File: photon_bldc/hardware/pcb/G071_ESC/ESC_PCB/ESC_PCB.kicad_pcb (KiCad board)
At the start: 4 copper layers, 36 x 16 mm, 69 parts, among them J2 Plus, J3 Minus, Q1 NMOS, Q2 NMOS, Q3 NMOS, Q4 NMOS, Q5 NMOS, Q6 NMOS, U1 STM32G071GBUx, U4 L78L06_SOT89

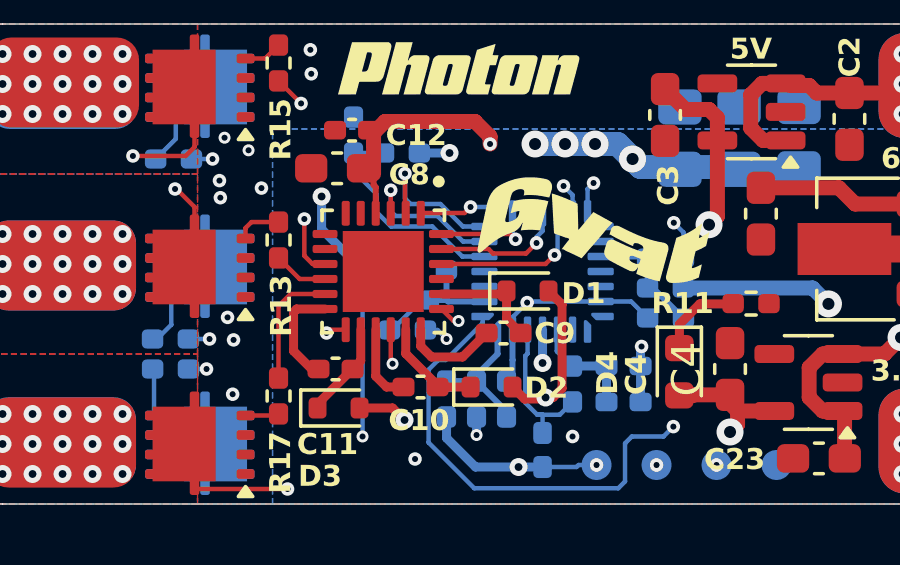
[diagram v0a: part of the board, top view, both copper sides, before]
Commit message: 11.05.2025r
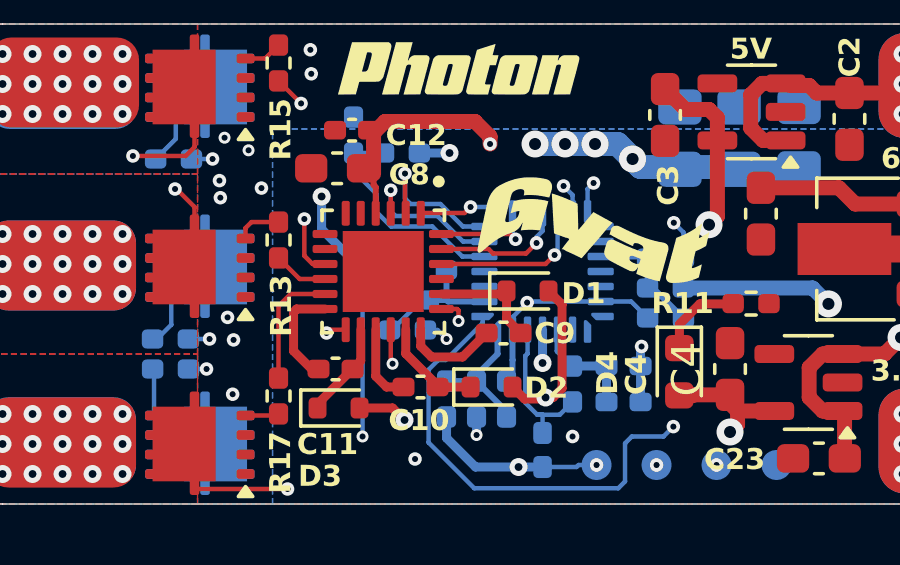
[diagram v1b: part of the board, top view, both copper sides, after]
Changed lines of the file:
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@@
 	)
 	(segment
-		(start 87.2 53.9)
-		(end 87.03 53.9)
+		(start 87.2 53.55)
+		(end 87.15 53.5)
 		(width 0.15)
 		(layer "F.Cu")
@@
 	)
 	(segment
-		(start 87.03 53.9)
+		(start 87.2 53.9)
+		(end 87.2 53.55)
+		(width 0.15)
+		(layer "F.Cu")
+		(net 14)
+	)
+	(segment
+		(start 87.15 53.5)
 		(end 86.63 53.5)
 		(width 0.15)

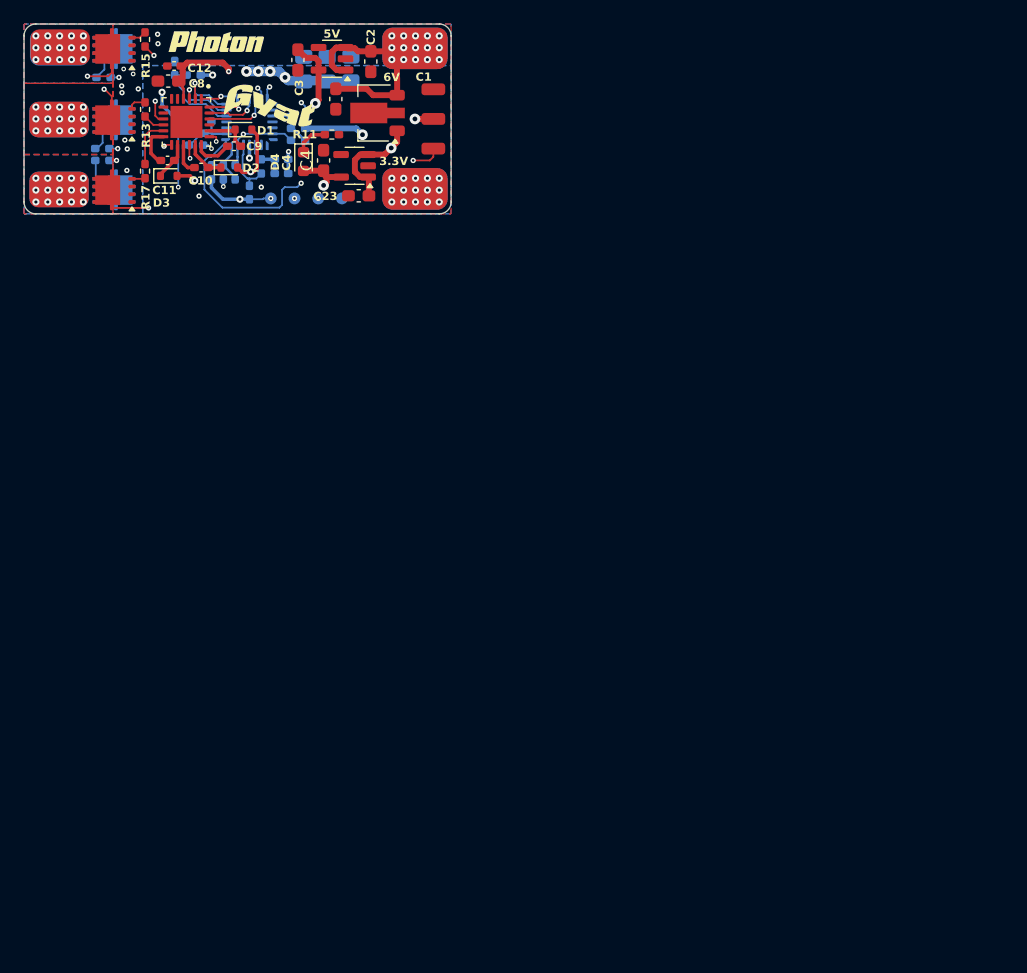
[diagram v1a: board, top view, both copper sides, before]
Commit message: esc
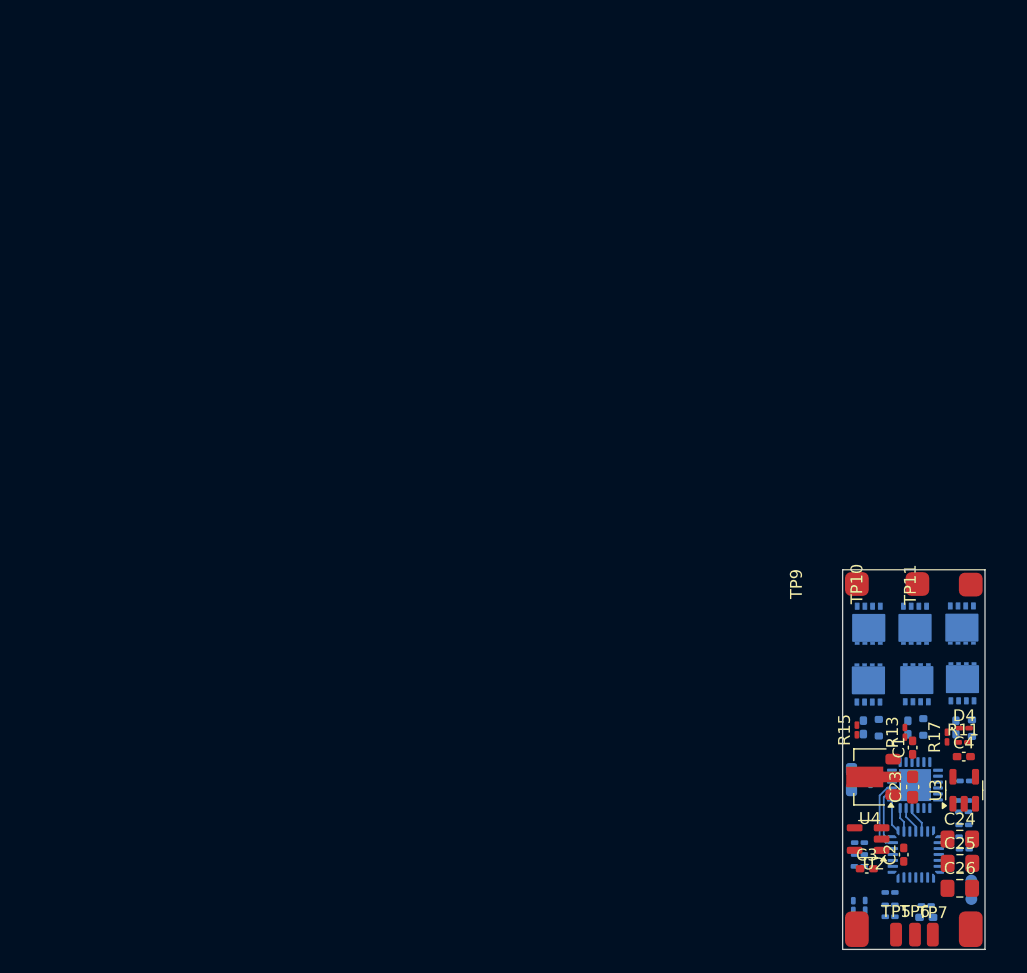
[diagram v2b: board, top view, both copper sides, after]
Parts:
- removed ? (x5): , 
- removed C5: 100nF, Capacitor_SMD:C_0402_1005Metric_Pad0.74x0.62mm_HandSolder
- removed G*** (x2): LOGO, LOGO
- removed R2: 10k, Resistor_SMD:R_0402_1005Metric_Pad0.72x0.64mm_HandSolder
- C1, C2, C3, C4: footprint Capacitor_SMD:C_0603_1608Metric_Pad1.08x0.95mm_HandSolder -> Capacitor_SMD:C_0402_1005Metric_Pad0.74x0.62mm_HandSolder
- C10, C11, C8, C9, D1, D2, D3, U6: moved to B.Cu
- C12: footprint Capacitor_SMD:C_0402_1005Metric_Pad0.74x0.62mm_HandSolder -> Capacitor_SMD:C_0201_0603Metric_Pad0.64x0.40mm_HandSolder; moved to B.Cu
- C24, C25, C26: moved to F.Cu
- C6: footprint Capacitor_SMD:C_0402_1005Metric_Pad0.74x0.62mm_HandSolder -> Capacitor_SMD:C_0201_0603Metric_Pad0.64x0.40mm_HandSolder
- D4: footprint LED_SMD:LED_0603_1608Metric -> LED_SMD:LED_0201_0603Metric_Pad0.64x0.40mm_HandSolder
- Q1, Q2, Q3: footprint Fortior Tech FD6288Q driver library:TSON-8(3.1x3.1) -> MOSFET_lib:NCEP3065
- Q4, Q5, Q6: footprint Fortior Tech FD6288Q driver library:TSON-8(3.1x3.1) -> MOSFET_lib:NCEP3065; moved to B.Cu
- R1, R10, R11, R12, R13, R14, R15, R16, R17, R18, R19, R3, R4, R5, R6, R7, R8, R9: footprint Resistor_SMD:R_0402_1005Metric_Pad0.72x0.64mm_HandSolder -> Resistor_SMD:R_0201_0603Metric_Pad0.64x0.40mm_HandSolder
- moved R14 93.7 mm to (150.3, 107.8), turned to 0 degrees
- moved R12 91.1 mm to (150.2, 109.5), turned to 0 degrees
- moved R16 91.0 mm to (150.2, 110.4), turned to 0 degrees
- moved R18 90.9 mm to (140.9, 118.3), turned to 90 degrees
- moved R19 90.0 mm to (141.9, 118.3), turned to -90 degrees
- moved C26 86.0 mm to (149.9, 116.8), turned to 0 degrees
- moved TP4 85.9 mm to (150.9, 121.0), turned to 180 degrees
- moved C25 85.6 mm to (149.9, 114.8), turned to 0 degrees
- moved C24 85.3 mm to (149.9, 112.7), turned to 0 degrees
- moved R4 84.9 mm to (144.0, 119.2), turned to 180 degrees
- moved Q6 84.0 mm to (142.2, 100.8)
- moved C12 84.0 mm to (142.3, 107.7), turned to 90 degrees
- moved TP11 83.8 mm to (150.8, 91.3)
- moved R6 83.6 mm to (141.4, 115.0)
- moved R15 83.6 mm to (141.2, 103.5)
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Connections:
- U1 pad 5: Net-(U1-PF2) -> unconnected-(U1-PF2-Pad5)
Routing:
- net GND: track 28.4 -> 0.00 mm, vias 26 -> 0
- net INPUT: track 28.2 -> 0.00 mm, vias 2 -> 0
- net PHASE_C: track 27.5 -> 0.00 mm, vias 17 -> 0
- net +6V: track 23.9 -> 0.00 mm, vias 4 -> 0
- net PHASE_B: track 20.4 -> 0.00 mm, vias 17 -> 0
- net +5V: track 17.5 -> 0.00 mm, vias 2 -> 0
- net VDC: track 17.2 -> 0.00 mm, vias 25 -> 0
- net SWDIO: track 14.6 -> 0.00 mm, vias 2 -> 0
- net +3.3V: track 13.9 -> 0.00 mm, vias 3 -> 0
- net PHASE_A: track 11.5 -> 0.00 mm, vias 17 -> 0
- net SWCLK: track 11.3 -> 0.00 mm, vias 2 -> 0
- net BEMF_REF: track 11.2 -> 0.00 mm, vias 2 -> 0
- net GHA: track 11.1 -> 0.00 mm, vias 2 -> 0
- net GHC: track 11.0 -> 0.00 mm, vias 2 -> 0
- net GHB: track 8.37 -> 0.00 mm, vias 2 -> 0
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- removed copper zone on B.Cu, net +3.3V
- removed copper zone on In2.Cu, net +6V
- removed copper zone on F.Cu, net GND
- removed copper zone on In1.Cu, net GND
- removed copper zone on B.Cu, net PHASE_A
- removed copper zone on F.Cu, net PHASE_A
- removed copper zone on B.Cu, net PHASE_B
- removed copper zone on F.Cu, net PHASE_B
- removed copper zone on B.Cu, net PHASE_C
- removed copper zone on F.Cu, net PHASE_C
- removed copper zone on B.Cu, net VDC
- removed copper zone on In1.Cu, net VDC
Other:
- board size 36 x 16 mm -> 12 x 32 mm
- board text removed: "+5V"
- board text removed: "3.3V"
- board text removed: "5V"
- board text removed: "6V"
- board text removed: "C1"
- board text removed: "C10"
- board text removed: "C11"
- board text removed: "C12"
- board text removed: "C2"
- board text removed: "C23"
- board text removed: "C24"
- board text removed: "C25"
- board text removed: "C26"
- board text removed: "C3"
- board text removed: "C4"
- board text removed: "C5"
- board text removed: "C6"
- board text removed: "C7"
- board text removed: "C8"
- board text removed: "C9"
- board text removed: "CLK"
- board text removed: "D1"
- board text removed: "D2"
- board text removed: "D3"
- board text removed: "D4"
- board text removed: "GND"
- board text removed: "PWM"
- board text removed: "R1"
- board text removed: "R10"
- board text removed: "R11"
- board text removed: "R12"
- board text removed: "R13"
- board text removed: "R14"
- board text removed: "R15"
- board text removed: "R16"
- board text removed: "R17"
- board text removed: "R18"
- board text removed: "R19"
- board text removed: "R2"
- board text removed: "R3"
- board text removed: "R4"
- board text removed: "R5"
- board text removed: "R6"
- board text removed: "R7"
- board text removed: "R8"
- board text removed: "R9"
- board text removed: "SWD"
- board text removed: "VDC"

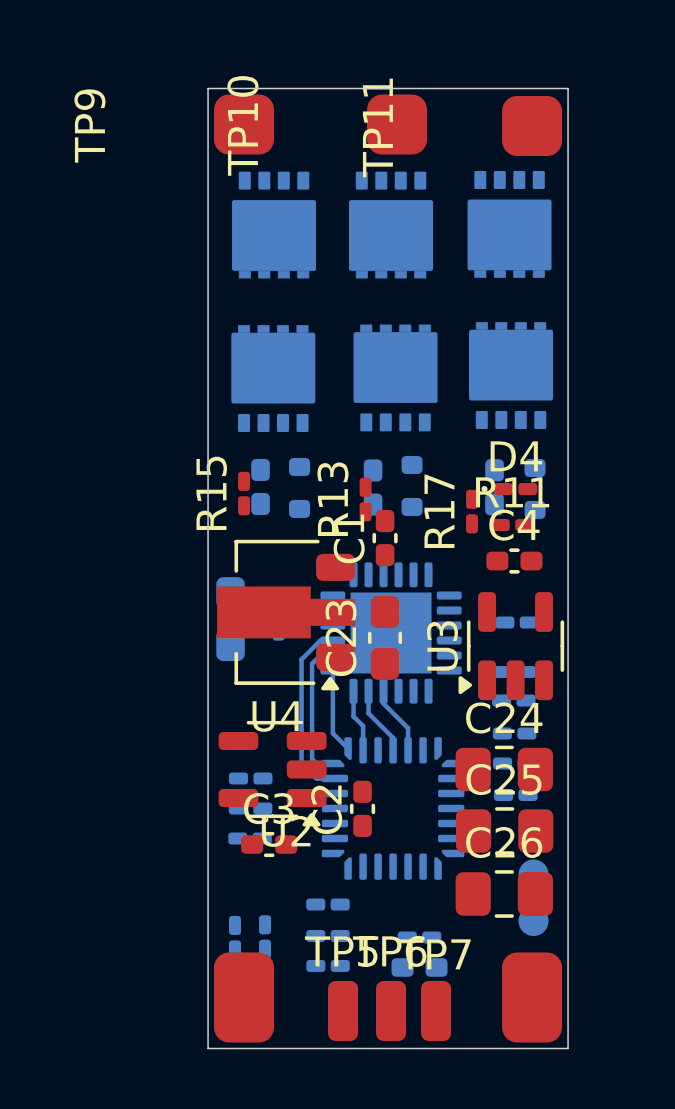
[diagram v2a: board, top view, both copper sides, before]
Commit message: oefvoj
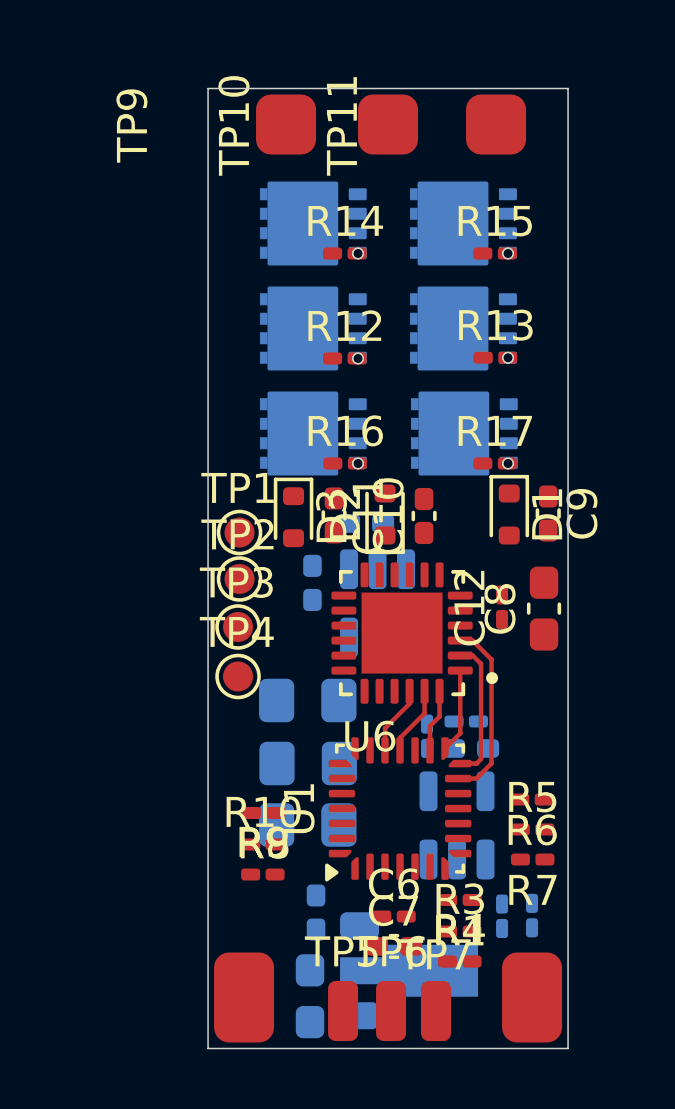
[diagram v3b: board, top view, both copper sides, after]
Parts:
- C1, C2, C23, C24, C25, C26, C3, C4, D4, R11, U2, U3, U4: moved to B.Cu
- C10, C11, C12, C6, C7, C8, C9, D1, D2, D3, R1, R10, R12, R14, R16, R3, R4, R5, R6, R7, R8, R9, TP1, TP2, TP3, TP4, U1, U6: moved to F.Cu
- moved TP4 15.1 mm to (141.0, 109.6), turned to 0 degrees
- moved TP3 15.1 mm to (141.0, 108.0), turned to 0 degrees
- moved TP1 15.0 mm to (141.1, 104.8), turned to 0 degrees
- moved TP2 15.0 mm to (141.1, 106.3), turned to 0 degrees
- moved R14 13.6 mm to (144.6, 95.5)
- moved U4 12.8 mm to (147.0, 119.4), turned to 0 degrees
- moved C1 12.7 mm to (143.6, 117.5), turned to -90 degrees
- moved C23 12.2 mm to (143.4, 120.3)
- moved R12 11.9 mm to (144.6, 99.0)
- moved R15 11.6 mm to (149.6, 95.5), turned to 0 degrees
- moved C8 10.5 mm to (151.2, 107.3)
- moved Q6 9.84 mm to (149.7, 94.5), turned to 90 degrees
- moved R7 9.78 mm to (150.8, 115.7)
- moved Q1 9.75 mm to (144.7, 101.5), turned to 90 degrees
- moved R16 9.70 mm to (144.6, 102.5)
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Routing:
- net Net-(Q6-G): vias 0 -> 1
- net Net-(Q5-G): vias 0 -> 1
- net Net-(Q4-G): vias 0 -> 1
- net Net-(Q3-G): vias 0 -> 1
- net Net-(Q2-G): vias 0 -> 1
- net Net-(Q1-G): vias 0 -> 1
